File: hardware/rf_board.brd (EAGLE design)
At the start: 109.9 x 68.6 mm, 31 parts, among them IC1 LM358MX, X3 KUSBVX

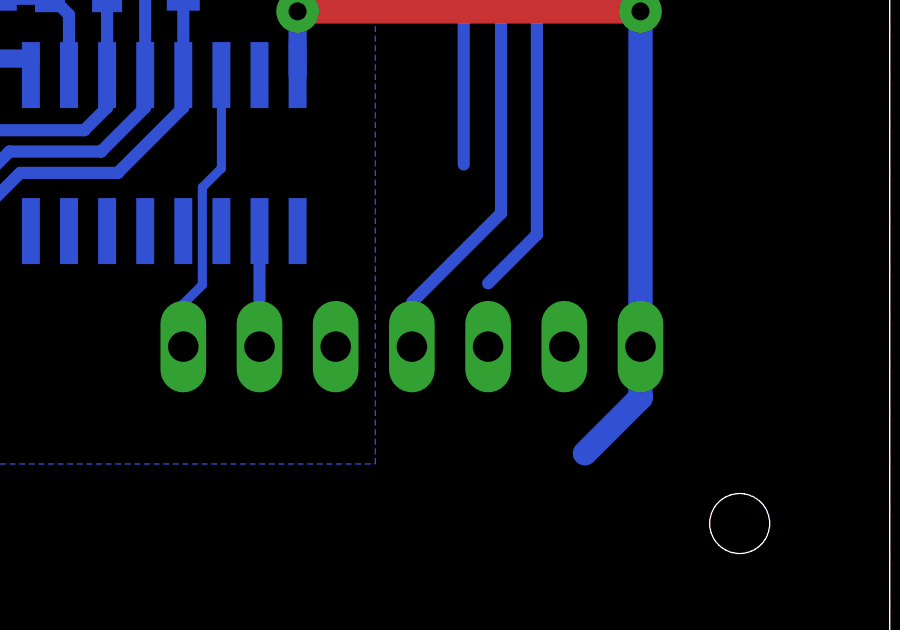
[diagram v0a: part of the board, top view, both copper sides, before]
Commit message: RF board update
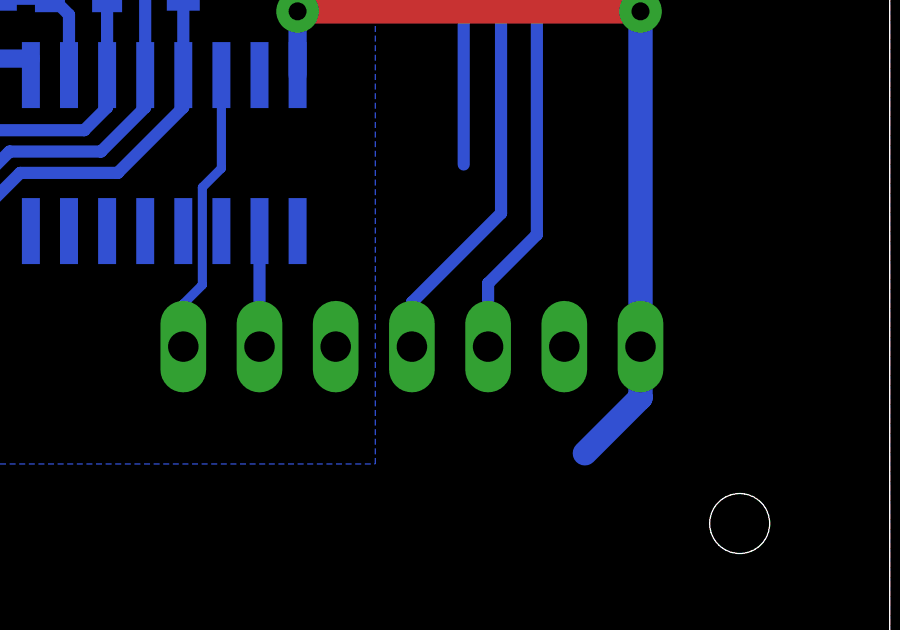
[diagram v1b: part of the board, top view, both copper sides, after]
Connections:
- removed net SCL: U$1.2
- removed net SDA: U$1.1
- net SCL1: now also U$1.2
- net SDA1: now also U$1.1
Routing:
- net SDA1: track 0.00 -> 72.8 mm, vias 0 -> 2
- net SCL1: track 0.00 -> 72.6 mm, vias 0 -> 2
- net SCL: track 71.1 -> 0.00 mm, vias 2 -> 0
- net SDA: track 70.6 -> 0.00 mm, vias 2 -> 0
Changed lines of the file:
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@@
 <contactref element="SV1" pad="3"/>
 <contactref element="JP2" pad="4"/>
+<contactref element="U$1" pad="2"/>
+<via x="59.055" y="55.5766" extent="1-16" drill="0.6" diameter="1.4224" shape="octagon"/>
+<wire x1="59.055" y1="55.5766" x2="61.881" y2="55.5766" width="0.6096" layer="16"/>
+<via x="96.901" y="55.5766" extent="1-16" drill="0.6" diameter="1.4224" shape="octagon"/>
+<wire x1="96.901" y1="55.5766" x2="96.901" y2="29.3116" width="0.4064" layer="16"/>
+<wire x1="96.901" y1="29.3116" x2="93.9292" y2="26.3398" width="0.4064" layer="16"/>
+<wire x1="59.055" y1="55.5766" x2="96.901" y2="55.5766" width="0.4064" layer="1"/>
+<wire x1="93.9292" y1="24.8666" x2="93.9292" y2="26.3398" width="0.4064" layer="16"/>
 <wire x1="63.119" y1="12.065" x2="93.9292" y2="24.8666" width="0" layer="19" extent="1-1"/>
 </signal>
@@
 <contactref element="SV1" pad="6"/>
 <contactref element="JP2" pad="3"/>
+<contactref element="U$1" pad="1"/>
+<via x="59.055" y="53.5766" extent="1-16" drill="0.6" diameter="1.4224" shape="octagon"/>
+<wire x1="59.055" y1="53.5766" x2="61.881" y2="53.5766" width="0.6096" layer="16"/>
+<via x="98.0948" y="54.3306" extent="1-16" drill="0.6" diameter="1.4224" shape="octagon"/>
+<wire x1="98.0948" y1="54.3306" x2="98.0948" y2="28.6004" width="0.4064" layer="16"/>
+<wire x1="98.0948" y1="28.6004" x2="96.4692" y2="26.9748" width="0.4064" layer="16"/>
+<wire x1="98.0948" y1="54.3306" x2="96.4184" y2="54.3306" width="0.4064" layer="1"/>
+<wire x1="96.4184" y1="54.3306" x2="95.885" y2="54.864" width="0.4064" layer="1"/>
+<wire x1="95.885" y1="54.864" x2="60.3424" y2="54.864" width="0.4064" layer="1"/>
+<wire x1="60.3424" y1="54.864" x2="59.055" y2="53.5766" width="0.4064" layer="1"/>
+<wire x1="96.4692" y1="24.8666" x2="96.4692" y2="26.9748" width="0.4064" layer="16"/>
 <wire x1="65.659" y1="9.525" x2="96.4692" y2="24.8666" width="0" layer="19" extent="1-1"/>
 </signal>
@@
 <wire x1="80.5948" y1="64.7198" x2="80.645" y2="64.77" width="0.34798125" layer="16"/>
 </signal>
-<signal name="SDA">
-<contactref element="U$1" pad="1"/>
-<via x="59.055" y="53.5766" extent="1-16" drill="0.6" diameter="1.4224" shape="octagon"/>
-<wire x1="59.055" y1="53.5766" x2="61.881" y2="53.5766" width="0.6096" layer="16"/>
-<via x="98.0948" y="54.3306" extent="1-16" drill="0.6" diameter="1.4224" shape="octagon"/>
-<wire x1="98.0948" y1="54.3306" x2="98.0948" y2="28.6004" width="0.4064" layer="16"/>
-<wire x1="98.0948" y1="28.6004" x2="96.4692" y2="26.9748" width="0.4064" layer="16"/>
-<wire x1="98.0948" y1="54.3306" x2="96.4184" y2="54.3306" width="0.4064" layer="1"/>
-<wire x1="96.4184" y1="54.3306" x2="95.885" y2="54.864" width="0.4064" layer="1"/>
-<wire x1="95.885" y1="54.864" x2="60.3424" y2="54.864" width="0.4064" layer="1"/>
-<wire x1="60.3424" y1="54.864" x2="59.055" y2="53.5766" width="0.4064" layer="1"/>
-</signal>
-<signal name="SCL">
-<contactref element="U$1" pad="2"/>
-<via x="59.055" y="55.5766" extent="1-16" drill="0.6" diameter="1.4224" shape="octagon"/>
-<wire x1="59.055" y1="55.5766" x2="61.881" y2="55.5766" width="0.6096" layer="16"/>
-<via x="96.901" y="55.5766" extent="1-16" drill="0.6" diameter="1.4224" shape="octagon"/>
-<wire x1="96.901" y1="55.5766" x2="96.901" y2="29.3116" width="0.4064" layer="16"/>
-<wire x1="96.901" y1="29.3116" x2="93.9292" y2="26.3398" width="0.4064" layer="16"/>
-<wire x1="59.055" y1="55.5766" x2="96.901" y2="55.5766" width="0.4064" layer="1"/>
-</signal>
 <signal name="CLK2">
